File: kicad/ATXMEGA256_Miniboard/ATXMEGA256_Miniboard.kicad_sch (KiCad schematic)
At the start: 26 parts, among them J1 2x5 IDC Socket, J10 1x2 Goldpin Header, J11 2x5 Goldpin Socket, J12 1x2 Goldpin Header, J13 USB micro B 2.0 Socket, J14 2x3 Goldpin Socket, J15 2x3 Goldpin Socket, J2 1x2 Screw Terminal, J3 2x3 Goldpin Header, J4 2x5 Goldpin Socket, J5 2x5 Goldpin Socket, J6 2x5 Goldpin Socket, J7 2x3 Goldpin Socket, J8 2x5 Goldpin Socket, J9 1x2 Goldpin Header, SW1 RESET, U1 ATXMEGA256A3B-AU, Y1 32.768 kHz, Y2 16 MHz

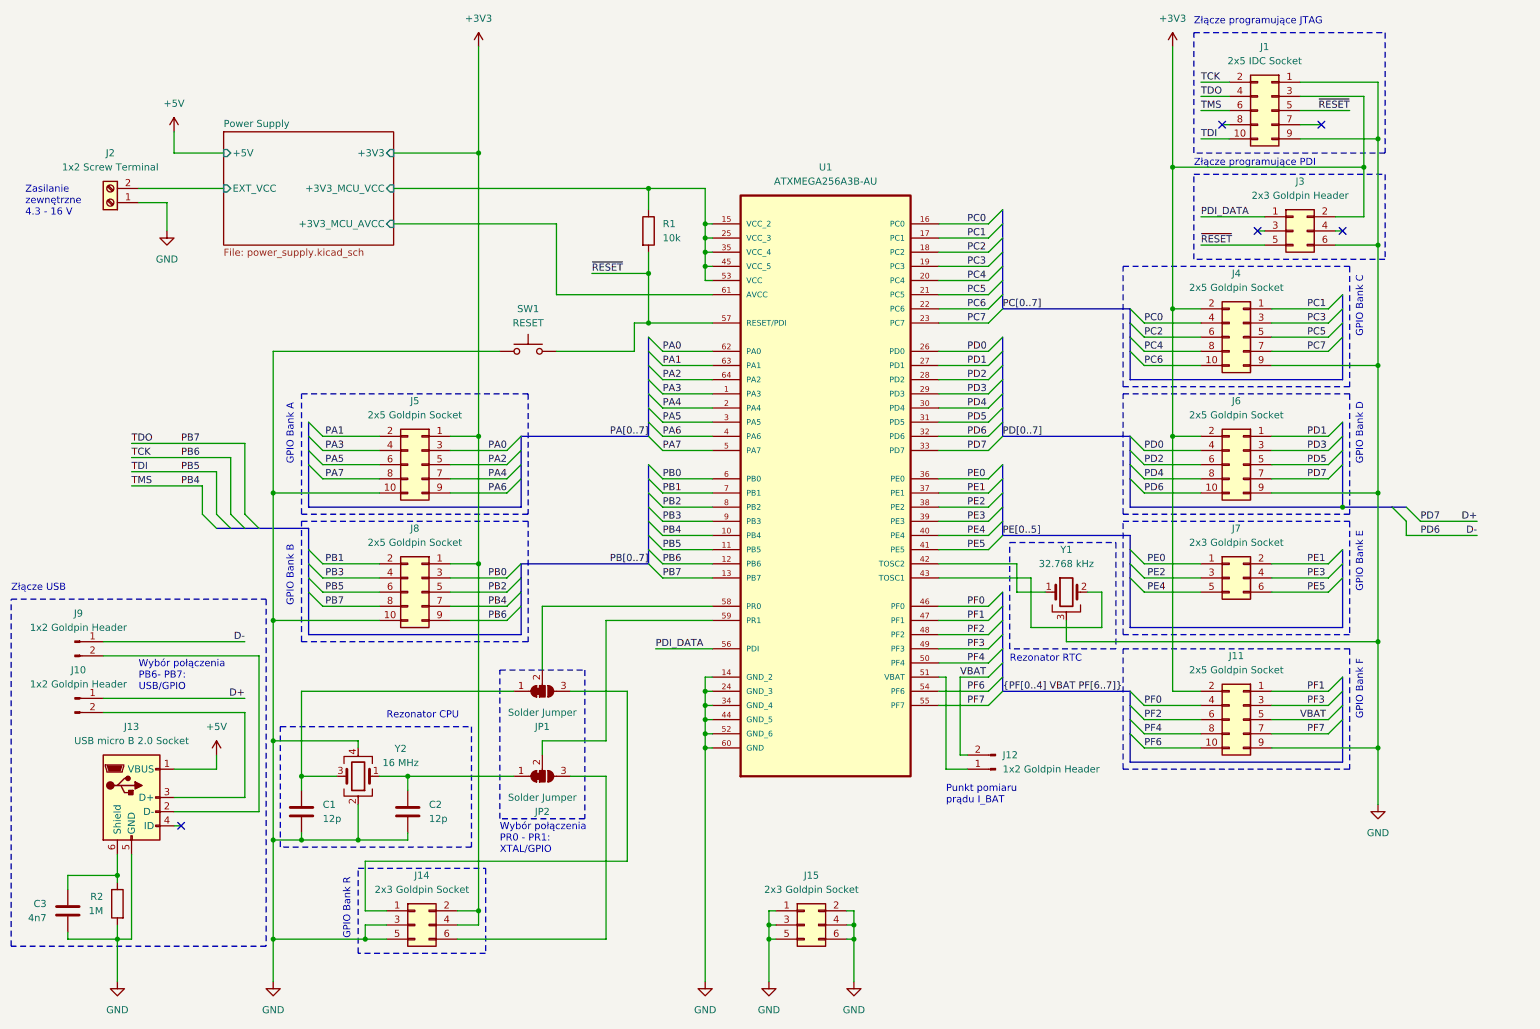
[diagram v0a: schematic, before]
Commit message: rev 1.1
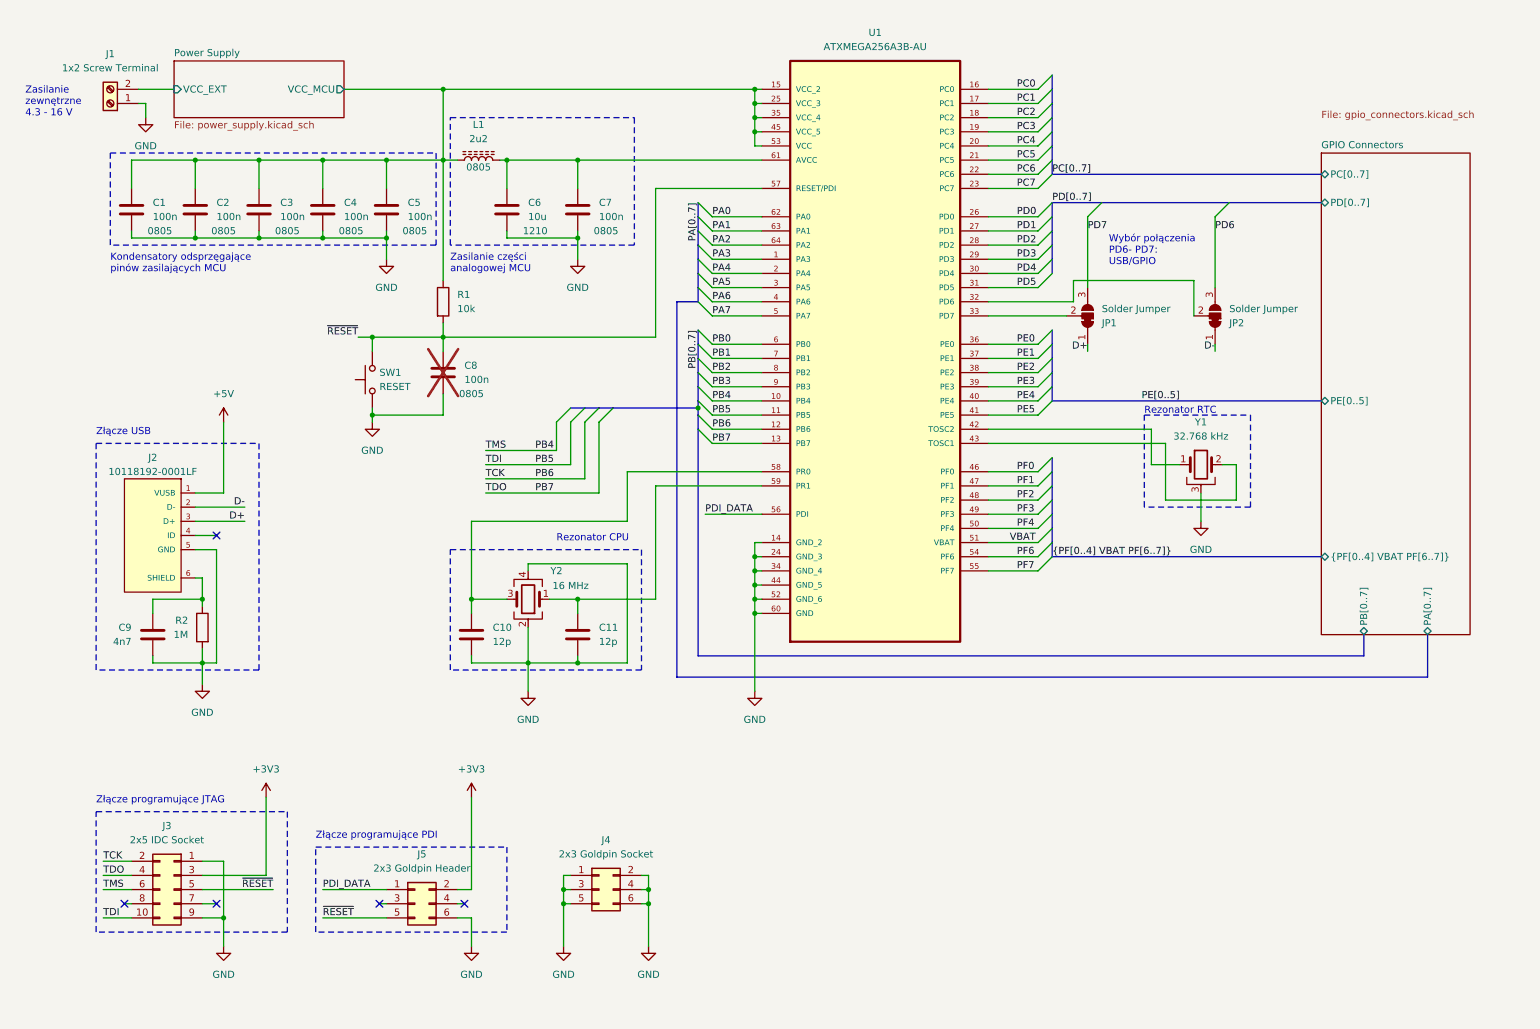
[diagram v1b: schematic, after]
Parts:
- removed J10, J12, J9: 1x2 Goldpin Header, Connector_PinHeader_2.54mm:PinHeader_1x02_P2.54mm_Vertical, symbol Connector:Conn_01x02_Pin
- removed J11, J4, J5, J6, J8: 2x5 Goldpin Socket, Connector_PinSocket_2.54mm:PinSocket_2x05_P2.54mm_Vertical_SMD, symbol Connector_Generic:Conn_02x05_Odd_Even
- removed J13: USB micro B 2.0 Socket, Connector_USB:USB_Micro-B_Amphenol_10118193-0001LF_Horizontal, symbol Connector:USB_B_Micro
- removed J14, J7: 2x3 Goldpin Socket, Connector_PinSocket_2.54mm:PinSocket_2x03_P2.54mm_Vertical_SMD, symbol Connector_Generic:Conn_02x03_Odd_Even
- removed J2: 1x2 Screw Terminal, TerminalBlock:TerminalBlock_bornier-2_P5.08mm, symbol Connector:Screw_Terminal_01x02
- added C1, C2, C3, C4, C5, C7, C8: 100n, Capacitor_SMD:C_0805_2012Metric_Pad1.18x1.45mm_HandSolder, symbol Device:C
- added C6: 10u, Capacitor_SMD:C_1210_3225Metric_Pad1.33x2.70mm_HandSolder, symbol Device:C
- added J1: 1x2 Screw Terminal, TerminalBlock:TerminalBlock_bornier-2_P5.08mm, symbol Connector:Screw_Terminal_01x02
- added J2: 10118192-0001LF, 10118192-0001LF:AMPHENOL_10118192-0001LF, symbol 10118192-0001LF:10118192-0001LF
- added L1: 2u2, Inductor_SMD:L_0805_2012Metric_Pad1.15x1.40mm_HandSolder, symbol Device:L_Ferrite
- JP1, JP2: footprint Jumper:SolderJumper-3_P1.3mm_Bridged12_Pad1.0x1.5mm_NumberLabels -> Jumper:SolderJumper-3_P1.3mm_Bridged12_RoundedPad1.0x1.5mm_NumberLabels
- renumbered C1 to C10, C2 to C11, C3 to C9, J1 to J3, J15 to J4, J3 to J5
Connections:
- net +5V: now also J2.1 (VUSB)
- net D+: now also JP1.1 (A), J2.3 (D+); no longer U1.33 (PD7)
- net D-: now also JP2.1 (A), J2.2 (D-); no longer U1.32 (PD6)
- net GND: now also C1.1, C2.1, C3.1, C4.1, C5.1, C6.1, C7.1, C8.1, J1.1 (Pin_1), J2.5 (GND)
- net VBAT: now also U1.51 (VBAT)
- net ~{RESET}: now also C8.2
- net PD7: now reaches JP1.3 (B)
- net PD6: now reaches JP2.3 (B)
- net at C9.2, R2.1: now also J2.6 (SHIELD)
- net at C10.2, Y2.3: now also U1.58 (PR0); no longer JP1.1 (A)
- net at JP1.2 (C): now also U1.33 (PD7); no longer U1.58 (PR0)
- net at C11.2, Y2.1: now also U1.59 (PR1); no longer JP2.1 (A)
- net at JP2.2 (C): now also U1.32 (PD6); no longer U1.59 (PR1)
- net Power Supply/+3V3_MCU_AVCC: no longer names the net of U1.61 (AVCC)
- net Power Supply/+3V3_MCU_AVCC: now also C6.2, C7.2, L1.2
- net Power Supply/+3V3_MCU_VCC renamed Power Supply/VCC_MCU
- net Power Supply/VCC_MCU: now also C1.2, C2.2, C3.2, C4.2, C5.2, L1.1
- new net Power Supply/VCC_EXT: J1.2 (Pin_2)
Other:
- added sheet GPIO Connectors (gpio_connectors.kicad_sch)
- sheet Power Supply ports: added VCC_EXT, VCC_MCU; removed +3V3, +3V3_MCU_AVCC, +3V3_MCU_VCC, +5V, EXT_VCC
- note added: "Kondensatory odsprzęgające pinów zasilających MCU"
- note added: "Wybór połączenia PD6- PD7: USB/GPIO"
- note added: "Zasilanie części analogowej MCU"
- note removed: "GPIO Bank A"
- note removed: "GPIO Bank B"
- note removed: "GPIO Bank C"
- note removed: "GPIO Bank D"
- note removed: "GPIO Bank E"
- note removed: "GPIO Bank F"
- note removed: "GPIO Bank R"
- note removed: "Punkt pomiaru prądu I_BAT"
- note removed: "Wybór połączenia PB6- PB7: USB/GPIO"
- note removed: "Wybór połączenia PR0 - PR1: XTAL/GPIO"
- moved on the sheet: C10, C11, C9, J3, J4, J5, R1, R2, SW1, U1, Y1, Y2
